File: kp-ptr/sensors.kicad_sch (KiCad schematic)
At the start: 37 parts, among them U2 MS560702BA03-50, U3 MMC5983MA, U4 H3LIS331, U5 L76-L, U6 NJG1156PCD, U7 LSM6DSO32

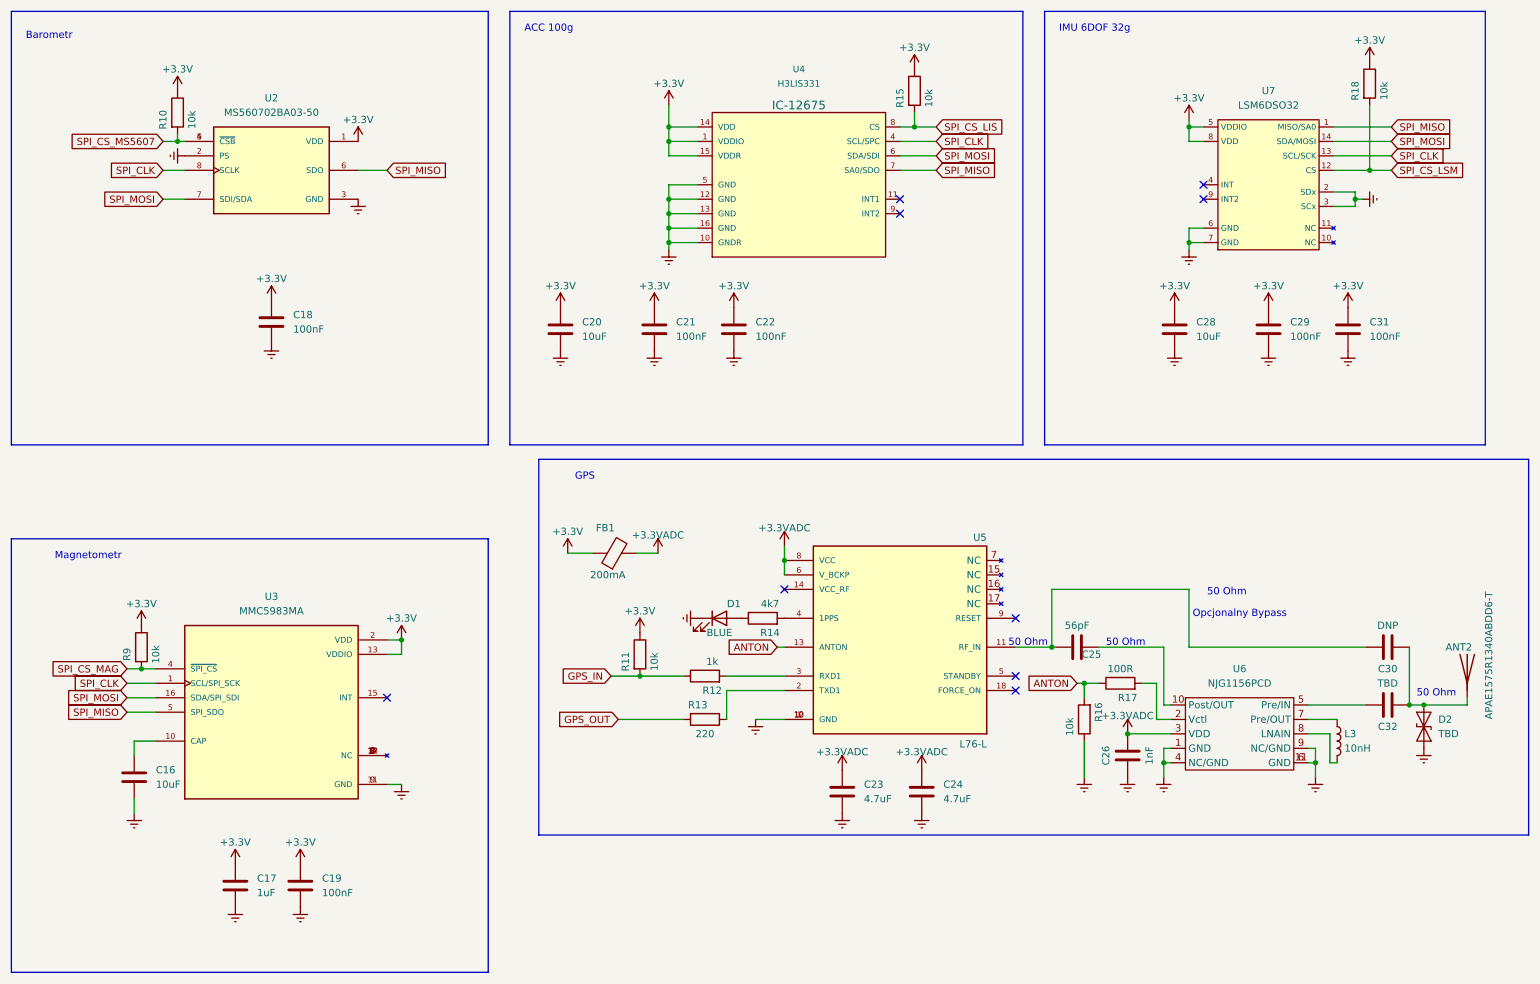
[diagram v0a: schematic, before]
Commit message: Release v0.1
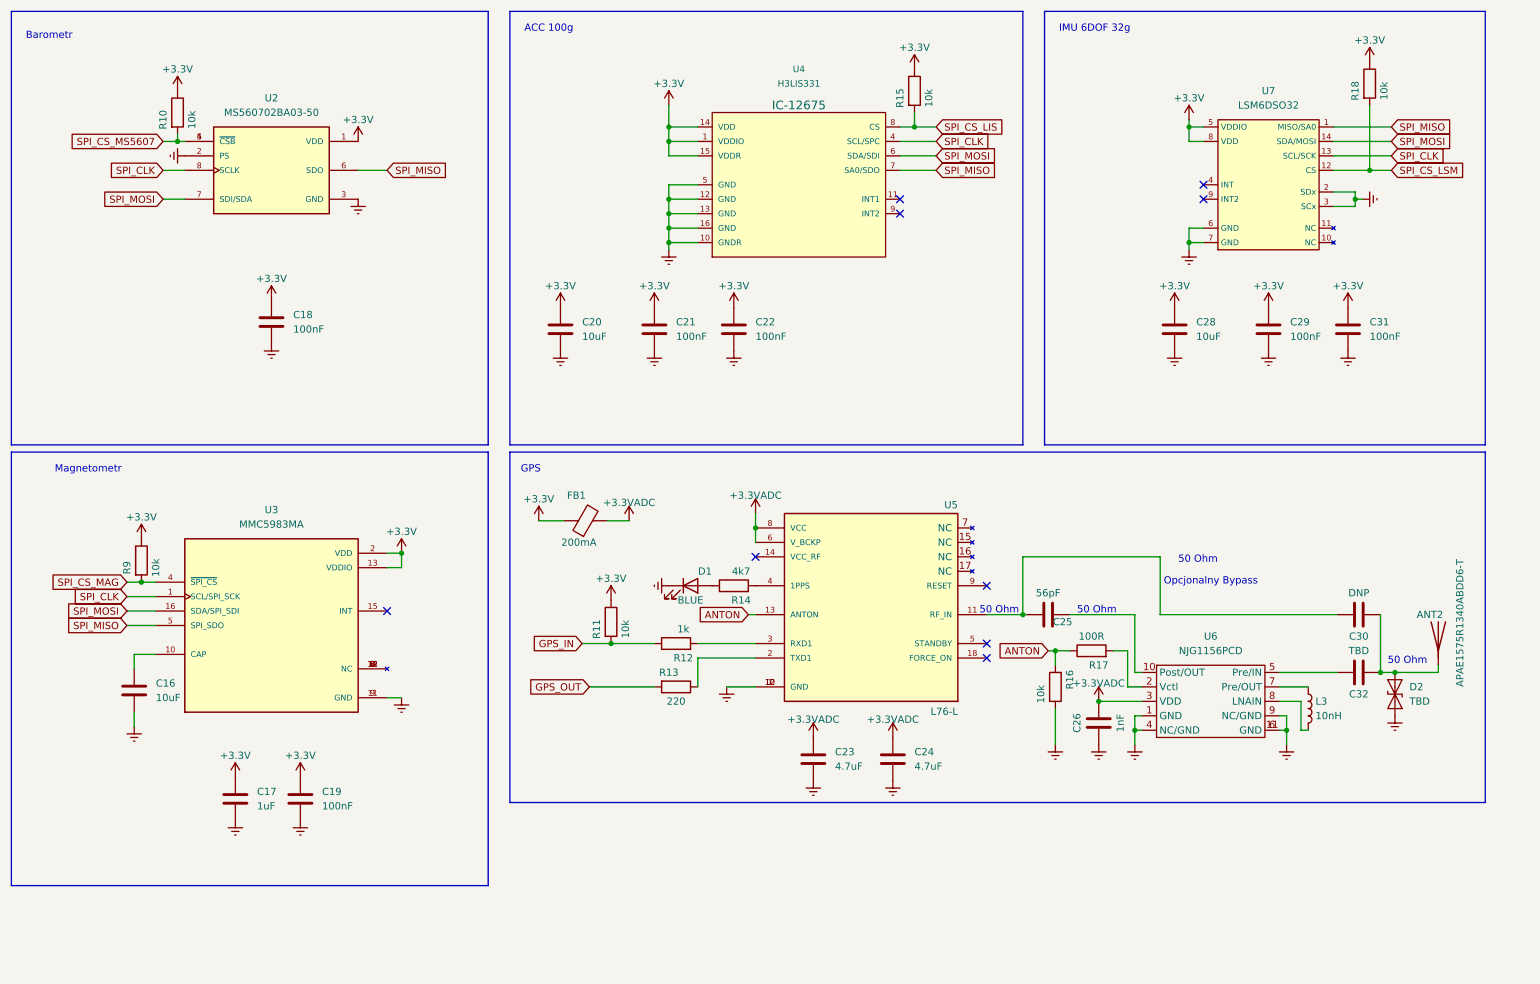
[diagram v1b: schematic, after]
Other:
- company: (none) -> Polskie Towarzystwo Rakietowe
- title: (none) -> KP-PTR
- moved on the sheet: ANT2, C16, C17, C19, C23, C24, C25, C26, C30, C32, D1, D2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
